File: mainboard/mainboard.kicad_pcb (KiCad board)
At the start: 2 copper layers, 80 x 100 mm, 68 parts, among them J1 Eurorack_Power, J2 Osc1_Socket, J3 Osc2_Socket, Q1 2N3906, Q2 2N3906, Q3 2N3904, Q4 2N3904, U1 40106, U2 TL074, U4 4070, U5 4520, U6 4015, U7 4015

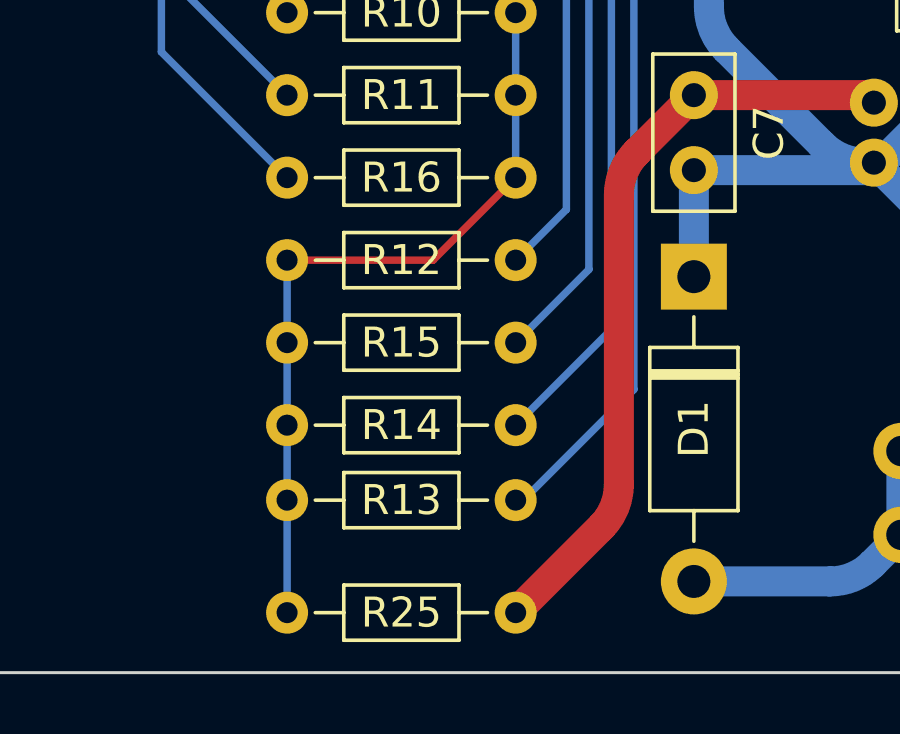
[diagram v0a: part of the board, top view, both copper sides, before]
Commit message: Updates to panel etc.
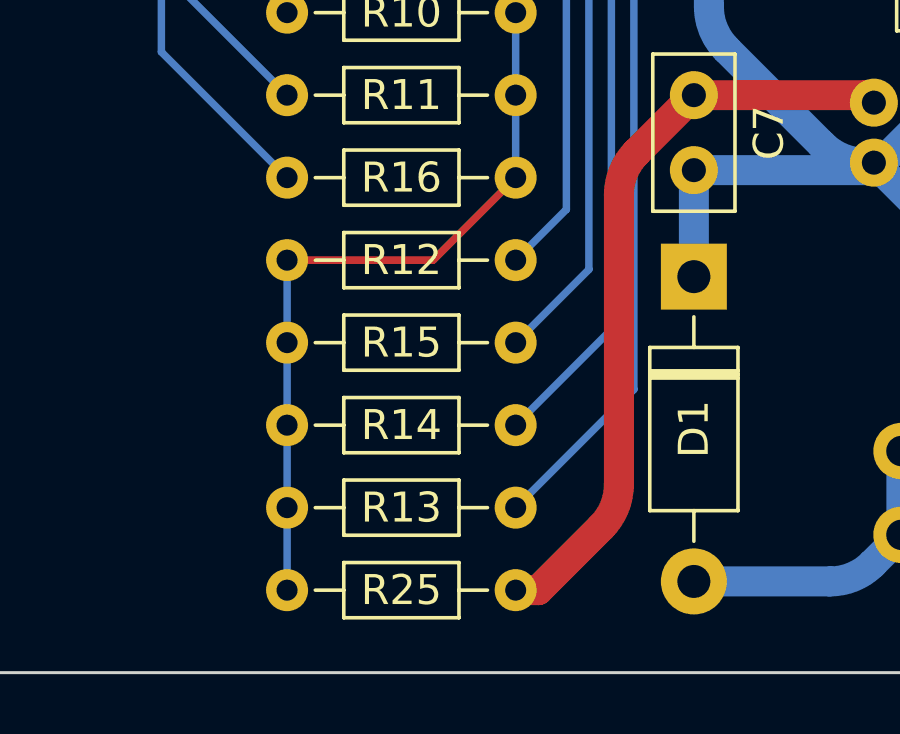
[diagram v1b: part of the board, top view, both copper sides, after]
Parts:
- moved R25 0.75 mm to (22.1, 97.2)
- moved R13 0.25 mm to (22.1, 94.5)
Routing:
- net Net-(R10-Pad2): track 44.2 -> 43.4 mm
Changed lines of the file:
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@@
   )
   (footprint "Resistor_THT:R_Axial_DIN0204_L3.6mm_D1.6mm_P7.62mm_Horizontal" (layer "F.Cu")
-    (at 22.06 98 180)
+    (at 22.06 97.25 180)
     (descr "Resistor, Axial_DIN0204 series, Axial, Horizontal, pin pitch=7.62mm, 0.167W, length*diameter=3.6*1.6mm^2, http://cdn-reichelt.de/documents/datenblatt/B400/1_4W%23YAG.pdf")
     (tags "Resistor Axial_DIN0204 series Axial Horizontal pin pitch 7.62mm 0.167W length 3.6mm diameter 1.6mm")
@@
   )
   (footprint "Resistor_THT:R_Axial_DIN0204_L3.6mm_D1.6mm_P7.62mm_Horizontal" (layer "F.Cu")
-    (at 22.06 94.25 180)
+    (at 22.06 94.5 180)
     (descr "Resistor, Axial_DIN0204 series, Axial, Horizontal, pin pitch=7.62mm, 0.167W, length*diameter=3.6*1.6mm^2, http://cdn-reichelt.de/documents/datenblatt/B400/1_4W%23YAG.pdf")
     (tags "Resistor Axial_DIN0204 series Axial Horizontal pin pitch 7.62mm 0.167W length 3.6mm diameter 1.6mm")
@@
   (segment (start 22.06 83.5) (end 22.06 80.75) (width 0.25) (layer "B.Cu") (net 37))
   (segment (start 22.06 80.75) (end 22.06 78) (width 0.25) (layer "B.Cu") (net 37))
+  (segment (start 14.44 94.5) (end 14.44 91.75) (width 0.25) (layer "B.Cu") (net 37))
   (segment (start 14.44 89) (end 14.44 86.25) (width 0.25) (layer "B.Cu") (net 37))
   (segment (start 14.44 91.75) (end 14.44 89) (width 0.25) (layer "B.Cu") (net 37))
-  (segment (start 14.44 94.25) (end 14.44 91.75) (width 0.25) (layer "B.Cu") (net 37))
-  (segment (start 14.44 98) (end 14.44 94.25) (width 0.25) (layer "B.Cu") (net 37))
+  (segment (start 14.44 97.25) (end 14.44 94.5) (width 0.25) (layer "B.Cu") (net 37))
   (segment (start 11.75 64.12) (end 11.75 75.31) (width 0.25) (layer "B.Cu") (net 38))
   (segment (start 14.5 61.37) (end 11.75 64.12) (width 0.25) (layer "B.Cu") (net 38))
@@
   (segment (start 74.75 20.85) (end 74.75 26.25) (width 0.25) (layer "F.Cu") (net 67))
   (segment (start 57.141422 35.25) (end 55.299511 37.091911) (width 0.25) (layer "F.Cu") (net 67))
+  (segment (start 25.501489 93.730134) (end 25.501489 84.079916) (width 1) (layer "F.Cu") (net 68))
   (segment (start 36.75 56) (end 38 56) (width 1) (layer "F.Cu") (net 68))
+  (segment (start 22.06 97.25) (end 22.81 97.25) (width 1) (layer "F.Cu") (net 68))
   (segment (start 41.25 36.5) (end 43.615 34.135) (width 1) (layer "F.Cu") (net 68))
-  (segment (start 25.5 93.731573) (end 25.5 84.078427) (width 1) (layer "F.Cu") (net 68))
-  (segment (start 26.085787 82.664213) (end 28 80.75) (width 1) (layer "F.Cu") (net 68))
   (segment (start 28 80.75) (end 33.75 80.75) (width 1) (layer "F.Cu") (net 68))
+  (segment (start 25.501489 84.079916) (end 25.5 84.078427) (width 1) (layer "F.Cu") (net 68))
   (segment (start 63.5 25.25) (end 57.500002 31.25) (width 1) (layer "F.Cu") (net 68))
   (segment (start 43.615 34.135) (end 43.8 34.135) (width 1) (layer "F.Cu") (net 68))
   (segment (start 63.5 25.24) (end 66.5 22.24) (width 1) (layer "F.Cu") (net 68))
+  (segment (start 22.81 97.25) (end 24.914214 95.145786) (width 1) (layer "F.Cu") (net 68))
   (segment (start 38 56) (end 41.25 52.75) (width 1) (layer "F.Cu") (net 68))
   (segment (start 66.5 22.24) (end 66.5 6.5) (width 1) (layer "F.Cu") (net 68))
   (segment (start 63.5 25.24) (end 63.5 25.25) (width 1) (layer "F.Cu") (net 68))
   (segment (start 28.5 44.25) (end 28.5 35.5) (width 1) (layer "F.Cu") (net 68))
+  (segment (start 25.5 93.731623) (end 25.501489 93.730134) (width 1) (layer "F.Cu") (net 68))
   (segment (start 33.75 80.75) (end 34 81) (width 1) (layer "F.Cu") (net 68))
-  (segment (start 22.06 98) (end 24.914214 95.145786) (width 1) (layer "F.Cu") (net 68))
   (segment (start 41.25 52.75) (end 41.25 36.5) (width 1) (layer "F.Cu") (net 68))
+  (segment (start 26.085787 82.664213) (end 28 80.75) (width 1) (layer "F.Cu") (net 68))
   (via (at 57.500002 31.25) (size 0.8) (drill 0.4) (layers "F.Cu" "B.Cu") (free) (net 68))
   (via (at 36.75 56) (size 0.8) (drill 0.4) (layers "F.Cu" "B.Cu") (free) (net 68))
-  (arc (start 25.5 93.731573) (mid 25.347759 94.49694) (end 24.914214 95.145786) (width 1) (layer "F.Cu") (net 68))
   (arc (start 25.5 84.078427) (mid 25.652241 83.31306) (end 26.085787 82.664213) (width 1) (layer "F.Cu") (net 68))
+  (arc (start 24.914214 95.145786) (mid 25.34776 94.496966) (end 25.5 93.731623) (width 1) (layer "F.Cu") (net 68))
   (segment (start 46 81) (end 51.75 81) (width 1) (layer "B.Cu") (net 68))
   (segment (start 14.5 71.53) (end 14.72 71.53) (width 1) (layer "B.Cu") (net 68))
